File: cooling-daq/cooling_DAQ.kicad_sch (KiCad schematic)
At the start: 58 parts, among them J1 Conn_02x10_Odd_Even, J1 USB_C_Receptacle_USB2.0_16P, J2 Conn_01x03_Pin, J3 Conn_01x02_Pin, J4 Conn_01x02_Pin, Q1 2N7002, Q2 2N7002, Q3 2N7002, SW1 SW_SPST, U1 STM32F103C8Tx, U2 AP2204K-ADJ, U3 AP2204K-ADJ, U6 SN65HVD256D, Y1 8M, Y2 32.768k

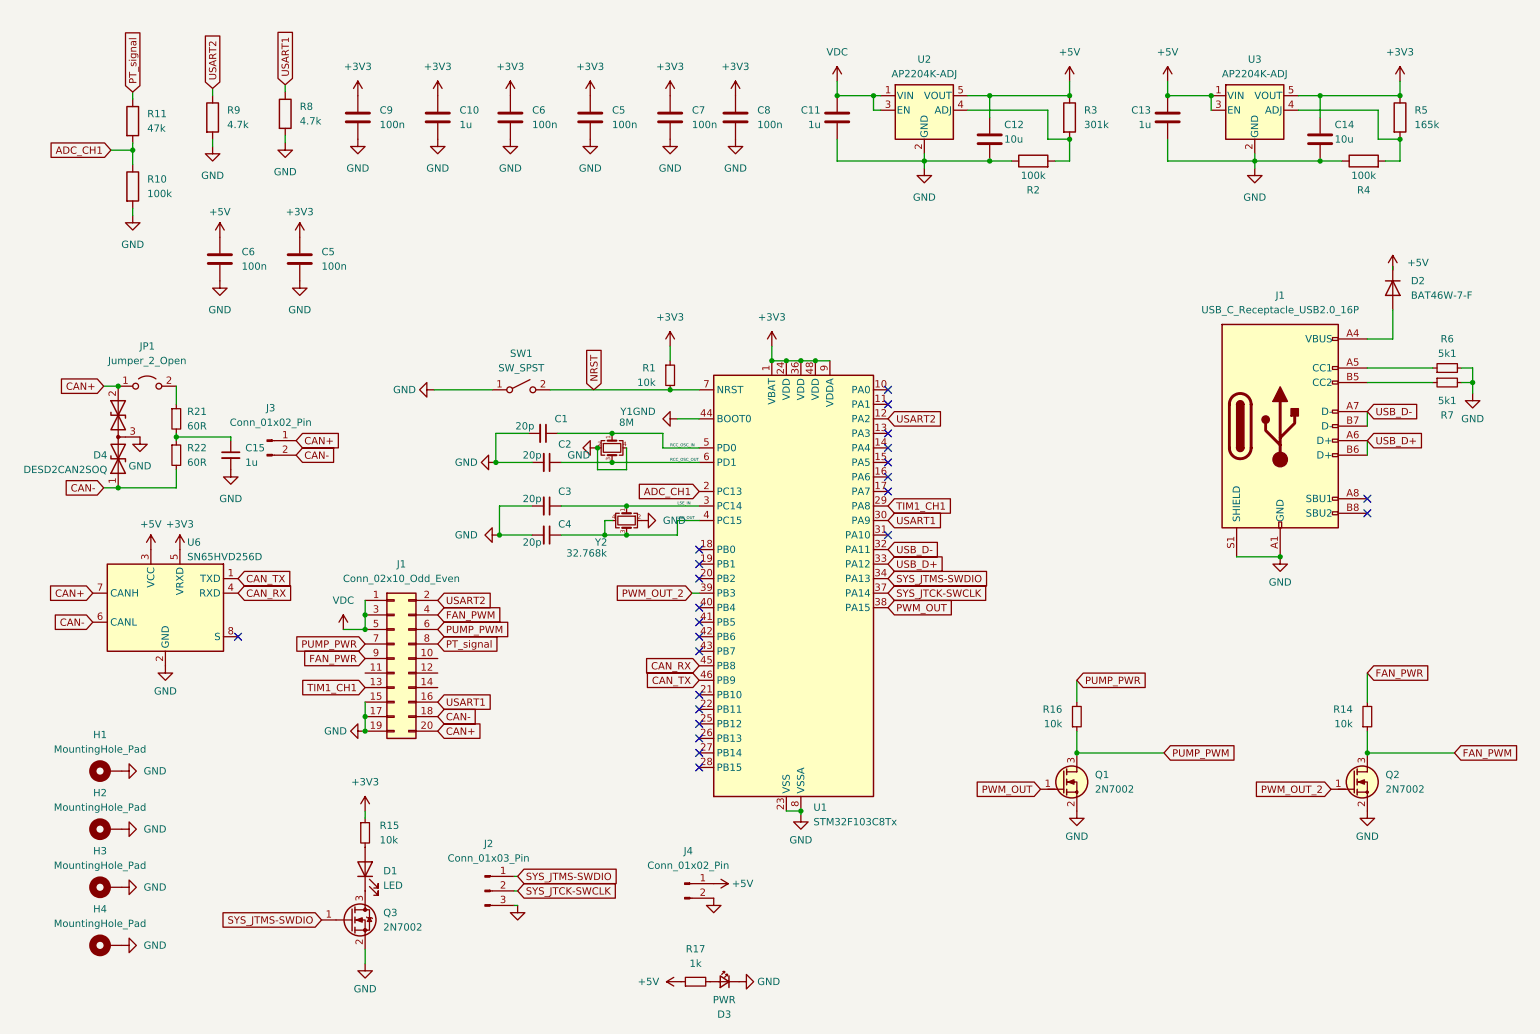
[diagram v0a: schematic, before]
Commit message: feat: redesign
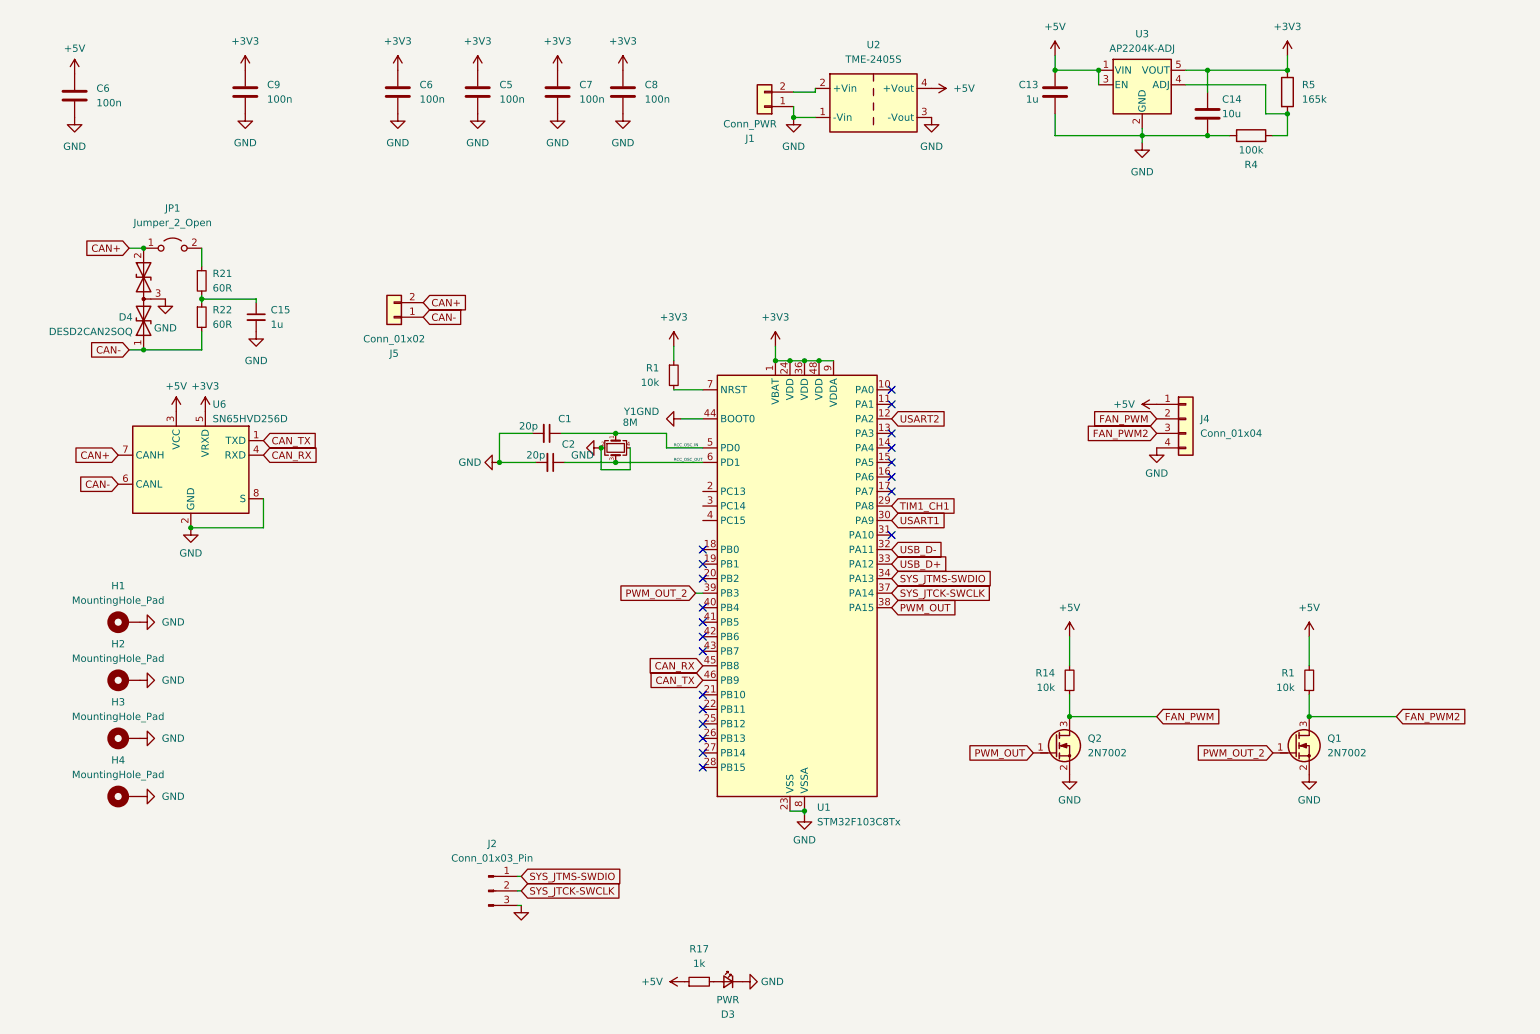
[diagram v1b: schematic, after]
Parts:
- removed C10, C11: 1u, Resistor_SMD:R_0603_1608Metric, symbol Device:C
- removed C12: 10u, Resistor_SMD:R_0805_2012Metric, symbol Device:C
- removed C3, C4: 20p, Capacitor_SMD:C_0603_1608Metric, symbol Device:C_Small
- removed C5: 100n, Resistor_SMD:R_0603_1608Metric, symbol Device:C
- removed D1: LED, LED_SMD:LED_0805_2012Metric, symbol Device:LED
- removed D2: BAT46W-7-F, Diode_SMD:D_SOD-123, symbol Diode:1N4148W
- removed J1: USB_C_Receptacle_USB2.0_16P, Connector_USB:USB_C_Receptacle_HRO_TYPE-C-31-M-12, symbol Connector:USB_C_Receptacle_USB2.0_16P
- removed J1: Conn_02x10_Odd_Even, Connector_PinHeader_2.54mm:PinHeader_2x10_P2.54mm_Vertical, symbol Connector_Generic:Conn_02x10_Odd_Even
- removed J3, J4: Conn_01x02_Pin, Connector_PinHeader_2.54mm:PinHeader_1x02_P2.54mm_Vertical, symbol Connector:Conn_01x02_Pin
- removed Q3: 2N7002, Package_TO_SOT_SMD:SOT-23, symbol Transistor_FET:2N7002
- removed R10, R2: 100k, Resistor_SMD:R_0603_1608Metric, symbol Device:R
- removed R11: 47k, Resistor_SMD:R_0603_1608Metric, symbol Device:R
- removed R15, R16: 10k, Resistor_SMD:R_0603_1608Metric, symbol Device:R_Small
- removed R3: 301k, Resistor_SMD:R_0603_1608Metric, symbol Device:R
- removed R6, R7: 5k1, Resistor_SMD:R_0603_1608Metric, symbol Device:R_Small
- removed R8, R9: 4.7k, Resistor_SMD:R_0603_1608Metric, symbol Device:R
- removed SW1: SW_SPST, Button_Switch_SMD:SW_SPST_FSMSM, symbol Switch:SW_SPST
- removed U2: AP2204K-ADJ, Package_TO_SOT_SMD:SOT-23-5, symbol Regulator_Linear:AP2204K-ADJ
- removed Y2: 32.768k, Crystal:Crystal_SMD_SeikoEpson_FA238-4Pin_3.2x2.5mm, symbol Device:Crystal_GND24_Small
- added J1: Conn_PWR, Connector_JST:JST_XH_B2B-XH-A_1x02_P2.50mm_Vertical, symbol Connector_Generic:Conn_01x02
- added J4: Conn_01x04, Connector_JST:JST_XH_B4B-XH-A_1x04_P2.50mm_Vertical, symbol Connector_Generic:Conn_01x04
- added J5: Conn_01x02, Connector_JST:JST_XH_B2B-XH-A_1x02_P2.50mm_Vertical, symbol Connector_Generic:Conn_01x02
- added R1: 10k, Resistor_SMD:R_0603_1608Metric, symbol Device:R_Small
- added U2: TME-2405S, Converter_DCDC:Converter_DCDC_TRACO_TME_24xxS_Single_THT, symbol Converter_DCDC:TME-2405S
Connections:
- net FAN_PWR is gone; now on net +5V: R14.2
- net +5V: now also J4.1 (Pin_1), R1.2, U2.4 (+Vout)
- net CAN+: now also J5.2 (Pin_2)
- net CAN-: now also J5.1 (Pin_1)
- net FAN_PWM: now also J4.2 (Pin_2)
- net GND: now also U6.8 (S), J1.1 (Pin_1), J4.4 (Pin_4), U2.1 (-Vin), U2.3 (-Vout)
- net PWM_OUT: now also Q2.1 (G); no longer Q1.1 (G)
- net PWM_OUT_2: now also Q1.1 (G); no longer Q2.1 (G)
- net ADC_CH1: no longer names the net of U1.2 (PC13)
- net LSE_IN: no longer names the net of U1.3 (PC14)
- net LSE_OUT: no longer names the net of U1.4 (PC15)
- net NRST: no longer names the net of R1.2, U1.7 (NRST)
- net PUMP_PWM renamed FAN_PWM2
- net FAN_PWM2: now also J4.3 (Pin_3), R1.1
- new net: J1.2 (Pin_2), U2.2 (+Vin)
- no-connect marks 24 -> 21
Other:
- moved on the sheet: C1, C13, C14, C15, C2, C5, C6, C7, C8, C9, D3, D4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
